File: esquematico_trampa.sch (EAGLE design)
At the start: 17 parts, among them U1 MICROCHIP_MCP3008-I-PMICROCHI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, U2 LM358PE3

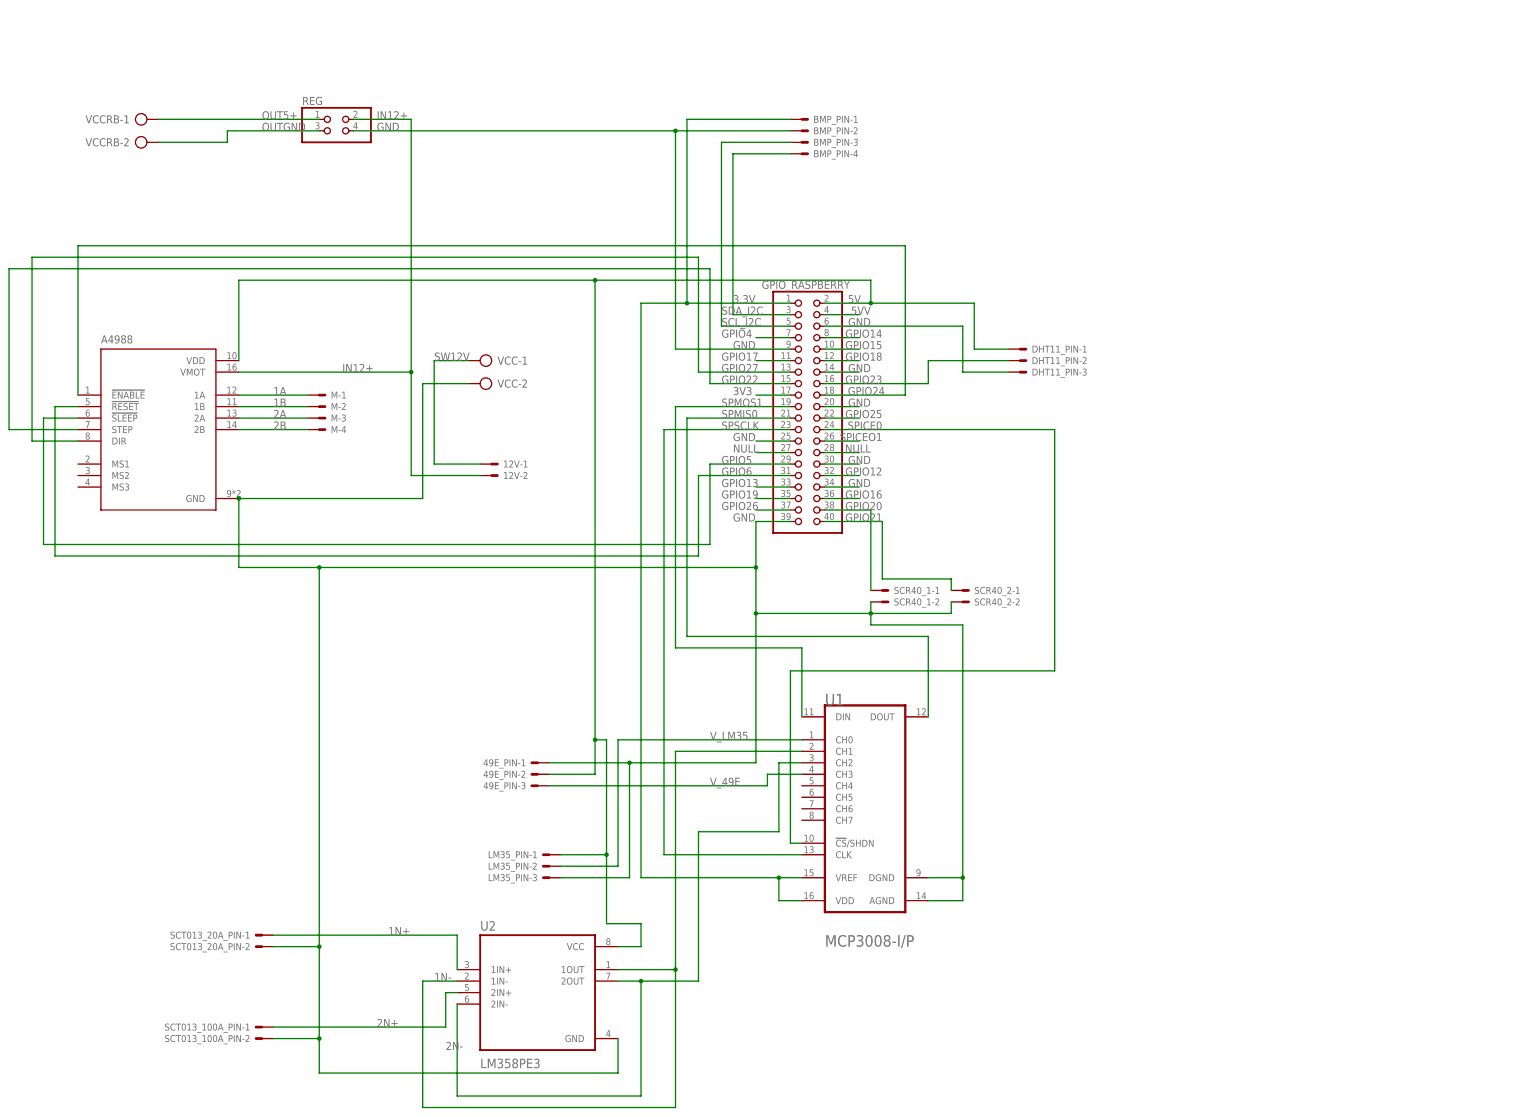
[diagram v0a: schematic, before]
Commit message: Esquemático más optimizado
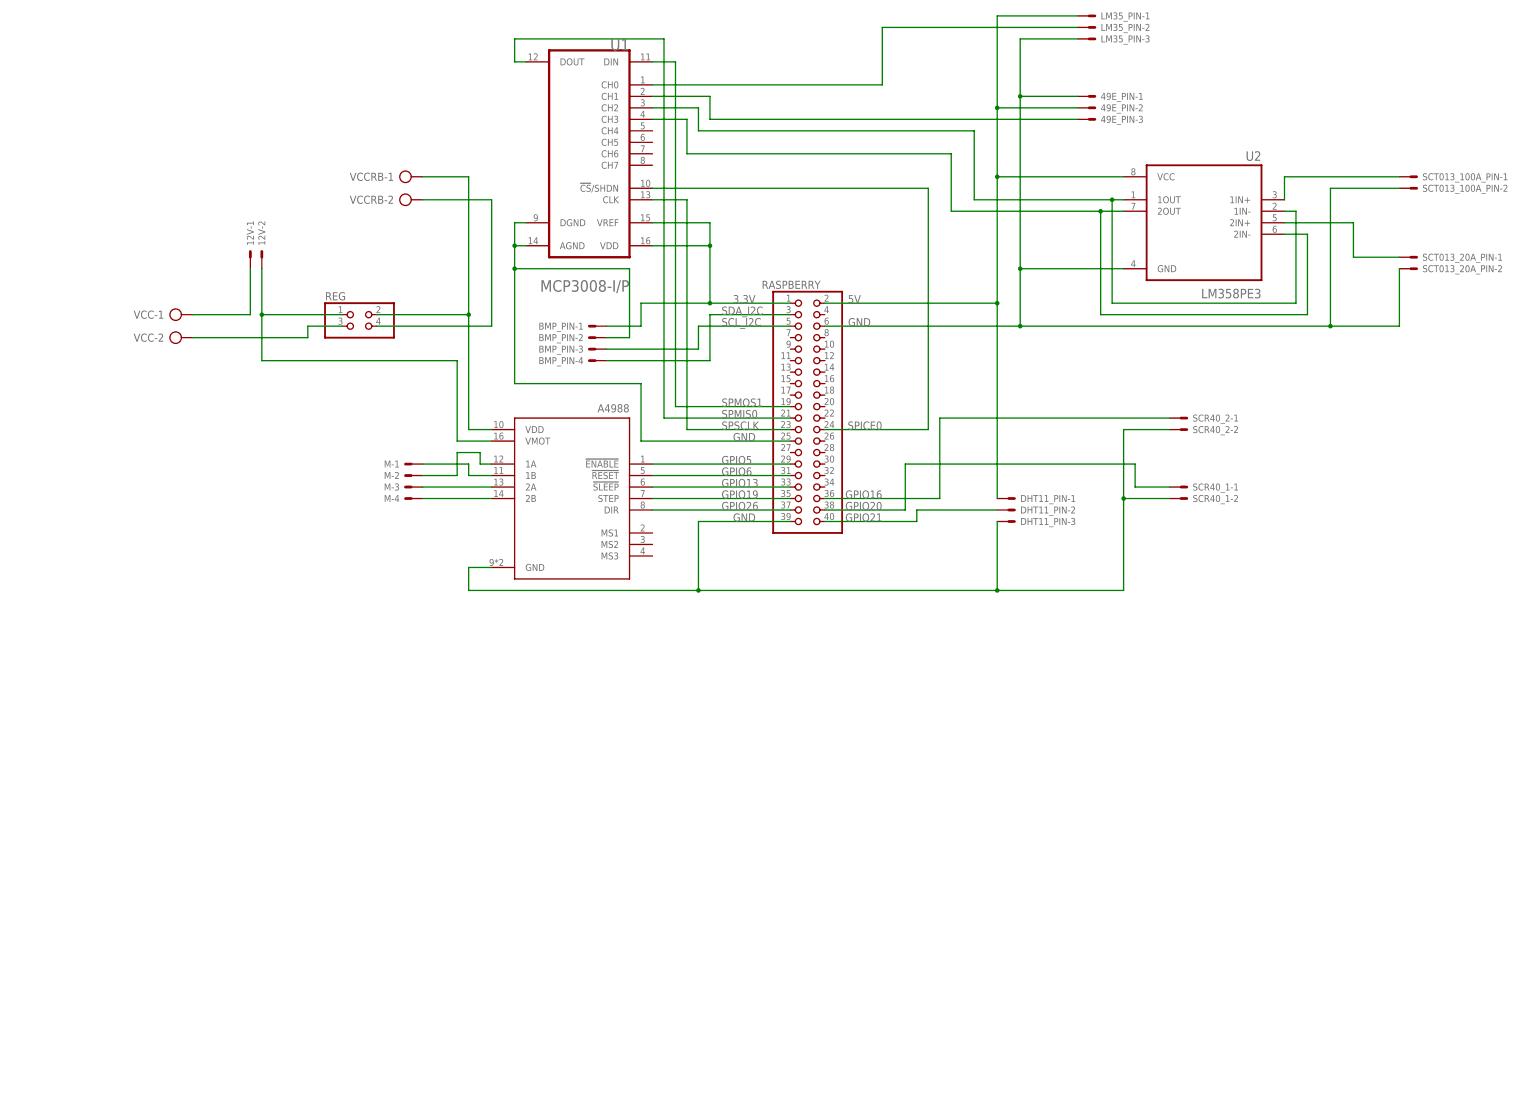
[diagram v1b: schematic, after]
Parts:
- renumbered GPIO_RASPBERRY to RASPBERRY
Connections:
- net 2A renamed N$3
- net 2B renamed N$4
- net SW12V renamed N$5
- net V_LM35 renamed N$10
- removed net 1A: A4988.1A, M-1.S
- removed net 1B: A4988.1B, M-2.S
- removed net 1N+: SCT013_20A_PIN-1.S, U2.1IN+
- removed net 1N-: U1.CH1, U2.1IN-, U2.1OUT
- removed net 2N+: SCT013_100A_PIN-1.S, U2.2IN+
- removed net 2N-: U1.CH2, U2.2IN-, U2.2OUT
- removed net 3V3: RASPBERRY.17
- removed net 5VV: RASPBERRY.4
- removed net GPIO12: RASPBERRY.32
- removed net GPIO14: RASPBERRY.8
- removed net GPIO15: RASPBERRY.10
- removed net GPIO17: RASPBERRY.11
- removed net GPIO18: RASPBERRY.12
- removed net GPIO22: A4988.STEP, RASPBERRY.15
- removed net GPIO23: DHT11_PIN-2.S, RASPBERRY.16
- removed net GPIO24: A4988.!ENABLE, RASPBERRY.18
- removed net GPIO25: RASPBERRY.22
- removed net GPIO27: A4988.DIR, RASPBERRY.13
- removed net GPIO4: RASPBERRY.7
- removed net IN12+: 12V-2.S, A4988.VMOT, REG.2
- removed net NULL: RASPBERRY.27, RASPBERRY.28
- removed net OUT5+: REG.1, VCCRB-1.KL
- removed net OUTGND: REG.3, VCCRB-2.KL
- removed net SPICEO1: RASPBERRY.26
- removed net V_49E: 49E_PIN-3.S, U1.CH3
- new net N$1: A4988.1B, M-1.S
- new net N$11: U1.CH2, U2.1IN-, U2.1OUT
- new net N$12: U1.CH3, U2.2IN-, U2.2OUT
- new net N$13: 49E_PIN-3.S, U1.CH1
- new net N$14: SCT013_100A_PIN-1.S, U2.1IN+
- new net N$16: SCT013_20A_PIN-1.S, U2.2IN+
- new net N$2: A4988.1A, M-2.S
- new net N$6: 12V-2.S, A4988.VMOT, REG.1
- new net N$7: REG.3, VCC-2.KL
- new net N$8: A4988.VDD, REG.2, VCCRB-1.KL
- new net N$9: REG.4, VCCRB-2.KL
- net 5V: no longer A4988.VDD
- net GND: no longer RASPBERRY.14, RASPBERRY.20, RASPBERRY.30, RASPBERRY.34, RASPBERRY.9, REG.4, VCC-2.KL
- net GPIO13: now also A4988.!SLEEP
- net GPIO16: now also SCR40_2-1.S
- net GPIO19: now also A4988.STEP
- net GPIO21: now also DHT11_PIN-2.S; no longer SCR40_2-1.S
- net GPIO26: now also A4988.DIR
- net GPIO5: now also A4988.!ENABLE; no longer A4988.!SLEEP
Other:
- moved on the sheet: 12V-1, 12V-2, 49E_PIN-1, 49E_PIN-2, 49E_PIN-3, A4988, BMP_PIN-1, BMP_PIN-2, BMP_PIN-3, BMP_PIN-4, DHT11_PIN-1, DHT11_PIN-2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
